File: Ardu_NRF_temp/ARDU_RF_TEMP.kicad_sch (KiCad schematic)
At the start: 34 parts, among them J1 DE9_Pins, J2 Conn_01x04_Socket, J3 Conn_01x04_Socket, J4 Conn_01x04_Socket, SW2 SW_Push, SW3 SW_Push, U1 NRF24L01_Breakout, U2 DHT11, U3 ESP-WROOM-32D, U4 NRF24L01_Breakout

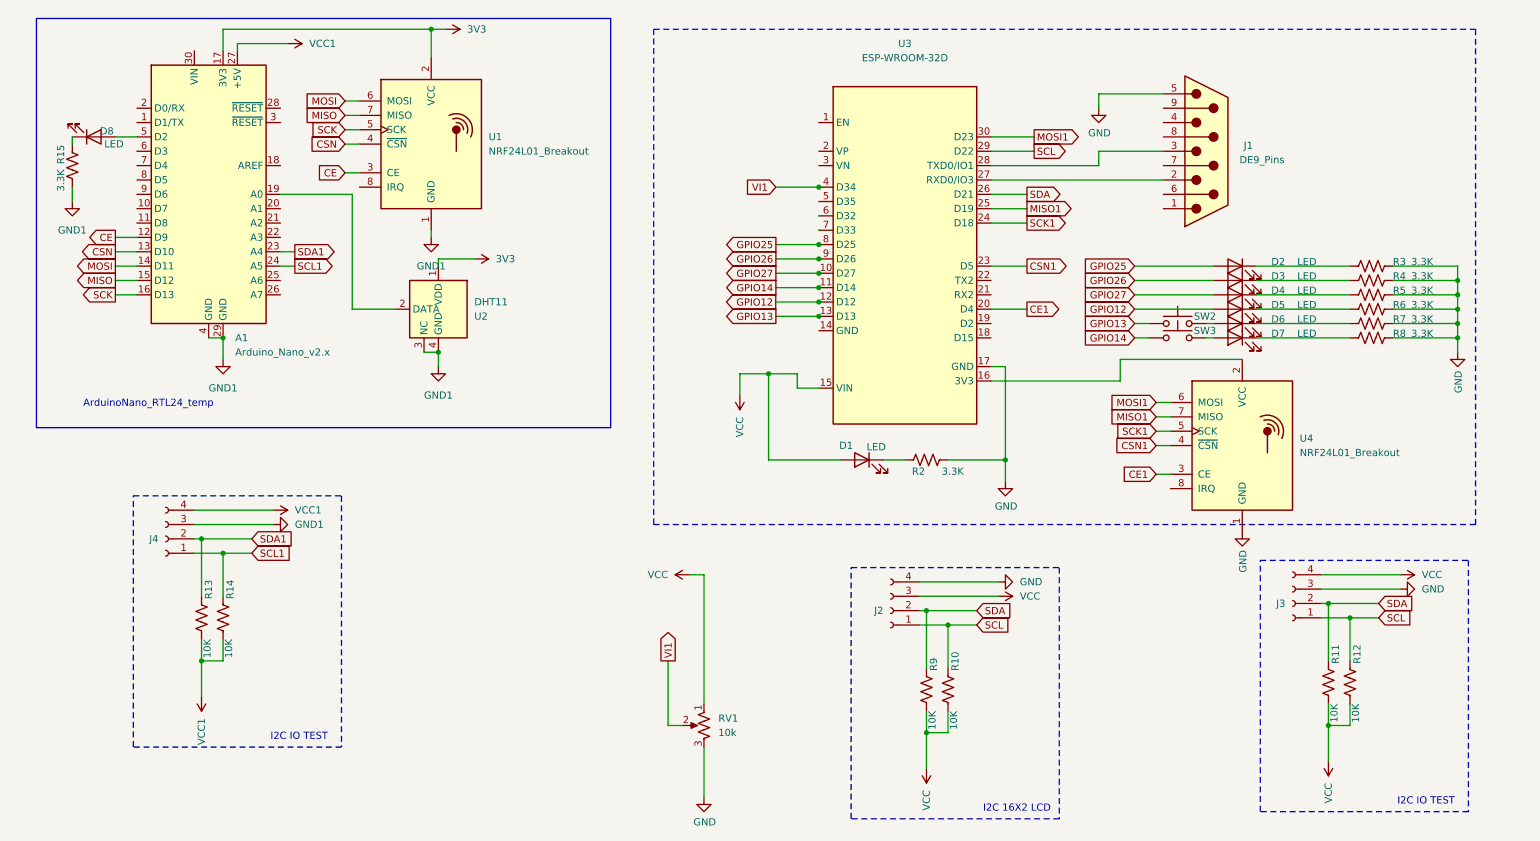
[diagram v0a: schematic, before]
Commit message: 5/21/25-1
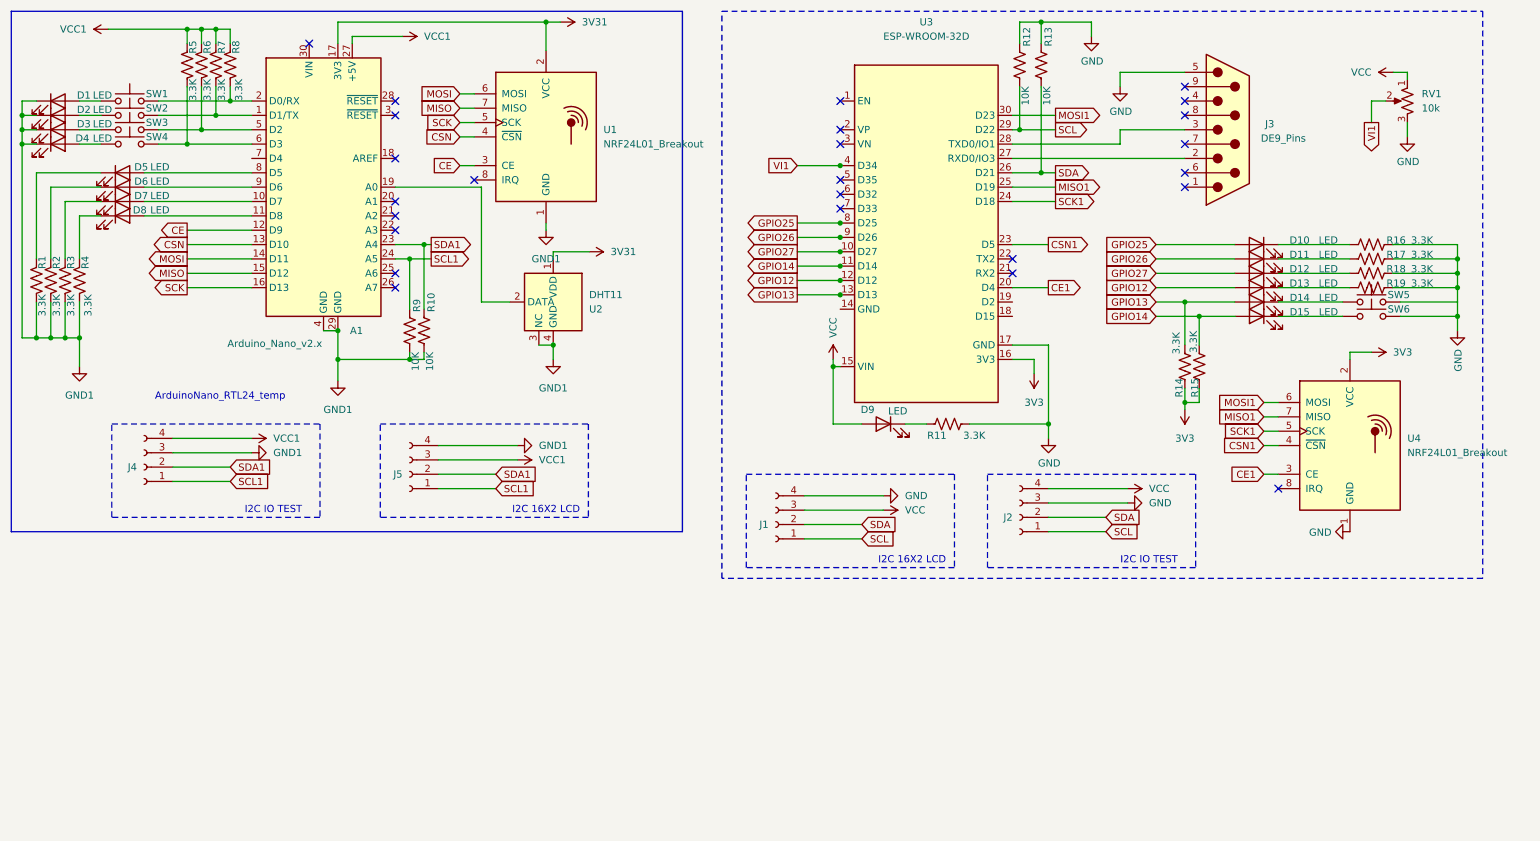
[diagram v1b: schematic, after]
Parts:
- removed J3: Conn_01x04_Socket, Add_New:CONN_PPPC041LGBN-RC_SUL, symbol Connector:Conn_01x04_Socket
- removed R11, R12: 10K, Resistor_THT:R_Axial_DIN0204_L3.6mm_D1.6mm_P5.08mm_Horizontal, symbol Device:R_US
- added D1, D15, D2, D3, D4, D5, D6: LED, LED_THT:LED_D3.0mm_Horizontal_O1.27mm_Z2.0mm, symbol Device:LED
- added J1, J5: Conn_01x04_Socket, Add_New:CONN_PPPC041LGBN-RC_SUL, symbol Connector:Conn_01x04_Socket
- added R1, R2, R3, R5, R6, R7, R8: 3.3K, Resistor_THT:R_Axial_DIN0207_L6.3mm_D2.5mm_P10.16mm_Horizontal, symbol Device:R_US
- added SW1, SW2, SW4, SW5: SW_Push, Button_Switch_SMD:SW_Tactile_SPST_NO_Straight_CK_PTS636Sx25SMTRLFS, symbol Switch:SW_Push
- J2: footprint Add_New:CONN_PPPC041LGBN-RC_SUL -> Add_New:CONN_PPTC041LFBN-RC_SUL
- R10: renamed from R14; footprint Resistor_THT:R_Axial_DIN0204_L3.6mm_D1.6mm_P5.08mm_Horizontal -> Resistor_THT:R_Axial_DIN0207_L6.3mm_D2.5mm_P10.16mm_Horizontal
- R11: renamed from R2; footprint Resistor_THT:R_Axial_DIN0204_L3.6mm_D1.6mm_P5.08mm_Horizontal -> Resistor_THT:R_Axial_DIN0207_L6.3mm_D2.5mm_P10.16mm_Horizontal
- R12: renamed from R9; footprint Resistor_THT:R_Axial_DIN0204_L3.6mm_D1.6mm_P5.08mm_Horizontal -> Resistor_THT:R_Axial_DIN0207_L6.3mm_D2.5mm_P10.16mm_Horizontal
- R13: renamed from R10; footprint Resistor_THT:R_Axial_DIN0204_L3.6mm_D1.6mm_P5.08mm_Horizontal -> Resistor_THT:R_Axial_DIN0207_L6.3mm_D2.5mm_P10.16mm_Horizontal
- R14: renamed from R7; footprint Resistor_THT:R_Axial_DIN0204_L3.6mm_D1.6mm_P5.08mm_Horizontal -> Resistor_THT:R_Axial_DIN0207_L6.3mm_D2.5mm_P10.16mm_Horizontal
- R15: renamed from R8; footprint Resistor_THT:R_Axial_DIN0204_L3.6mm_D1.6mm_P5.08mm_Horizontal -> Resistor_THT:R_Axial_DIN0207_L6.3mm_D2.5mm_P10.16mm_Horizontal
- R16: renamed from R3; footprint Resistor_THT:R_Axial_DIN0204_L3.6mm_D1.6mm_P5.08mm_Horizontal -> Resistor_THT:R_Axial_DIN0207_L6.3mm_D2.5mm_P10.16mm_Horizontal
- R17: renamed from R4; footprint Resistor_THT:R_Axial_DIN0204_L3.6mm_D1.6mm_P5.08mm_Horizontal -> Resistor_THT:R_Axial_DIN0207_L6.3mm_D2.5mm_P10.16mm_Horizontal
- R18: renamed from R5; footprint Resistor_THT:R_Axial_DIN0204_L3.6mm_D1.6mm_P5.08mm_Horizontal -> Resistor_THT:R_Axial_DIN0207_L6.3mm_D2.5mm_P10.16mm_Horizontal
- R19: renamed from R6; footprint Resistor_THT:R_Axial_DIN0204_L3.6mm_D1.6mm_P5.08mm_Horizontal -> Resistor_THT:R_Axial_DIN0207_L6.3mm_D2.5mm_P10.16mm_Horizontal
- R4: renamed from R15; footprint Resistor_THT:R_Axial_DIN0204_L3.6mm_D1.6mm_P5.08mm_Horizontal -> Resistor_THT:R_Axial_DIN0207_L6.3mm_D2.5mm_P10.16mm_Horizontal
- R9: renamed from R13; footprint Resistor_THT:R_Axial_DIN0204_L3.6mm_D1.6mm_P5.08mm_Horizontal -> Resistor_THT:R_Axial_DIN0207_L6.3mm_D2.5mm_P10.16mm_Horizontal
- RV1: footprint Potentiometer_THT:Potentiometer_Alps_RK09Y11_Single_Horizontal -> Potentiometer_THT:Potentiometer_Alps_RK163_Single_Horizontal
- SW3: footprint Button_Switch_THT:SW_DIP_SPSTx01_Slide_6.7x4.1mm_W7.62mm_P2.54mm_LowProfile -> Button_Switch_SMD:SW_Tactile_SPST_NO_Straight_CK_PTS636Sx25SMTRLFS
- SW6: renamed from SW2; footprint Button_Switch_THT:SW_DIP_SPSTx01_Slide_6.7x4.1mm_W7.62mm_P2.54mm_LowProfile -> Button_Switch_SMD:SW_Tactile_SPST_NO_Straight_CK_PTS636Sx25SMTRLFS
- renumbered D2 to D10, D3 to D11, D4 to D12, D5 to D13, D6 to D14, D1 to D9, J1 to J3
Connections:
- net 3V3: now also R14.1, R15.1, U4.2 (VCC); no longer A1.17 (3V3), U1.2 (VCC), U2.1 (VDD)
- net GND: now also J2.3 (Pin_3), R12.1, R13.1, SW6.2, J1.4 (Pin_4); no longer J2.4 (Pin_4), R14.2, R15.2
- net GND1: now also R10.2, R9.2, D1.1 (K), D2.1 (K), D3.1 (K), D4.1 (K), J5.4 (Pin_4), R1.2, R2.2, R3.2
- net GPIO13: now also D14.2 (A), R14.2; no longer SW6.1
- net GPIO14: now also R15.2, D15.2 (A); no longer SW3.1
- net SCL: now also R12.2, J1.1 (Pin_1); no longer R13.1
- net SCL1: now also R9.1, J5.1 (Pin_1); no longer R10.1
- net SDA: now also R13.2, J1.2 (Pin_2); no longer R12.1
- net SDA1: now also R10.1, J5.2 (Pin_2); no longer R9.1
- net VCC: now also J2.4 (Pin_4), J1.3 (Pin_3); no longer J2.3 (Pin_3), R12.2, R13.2
- net VCC1: now also J5.3 (Pin_3), R5.1, R6.1, R7.1, R8.1; no longer R10.2, R9.2
- net at D7.2 (A): now also A1.10 (D7); no longer SW3.2
- net at D7.1 (K): now also R3.1; no longer R15.1
- net at A1.1 (D1/TX): now also R7.2, SW2.2
- net at A1.11 (D8): now also D8.2 (A)
- net at A1.2 (D0/RX): now also R8.2, SW1.2
- net at A1.5 (D2): now also SW3.2, R6.2; no longer D8.2 (A)
- net at A1.6 (D3): now also R5.2, SW4.2
- net at A1.8 (D5): now also D5.2 (A)
- net at A1.9 (D6): now also D6.2 (A)
- net at D14.1 (K): now also SW5.1; no longer R14.1
- net at U3.16 (3V3): no longer U4.2 (VCC)
- new net: D6.1 (K), R2.1
- new net: D3.2 (A), SW3.1
- new net: D5.1 (K), R1.1
- new net: D15.1 (K), SW6.1
- new net: D4.2 (A), SW4.1
- new net: D1.2 (A), SW1.1
- new net: D2.2 (A), SW2.1
- new net 3V31: A1.17 (3V3), U1.2 (VCC), U2.1 (VDD)
- no-connect marks 0 -> 25
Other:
- moved on the sheet: A1, D10, D11, D12, D13, D14, D8, D9, J3, J4, R10, R11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
